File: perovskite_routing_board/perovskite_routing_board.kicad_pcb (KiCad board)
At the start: 4 copper layers, 57 x 52.2 mm, 10 parts, among them J1 G125-MH12605M4R, J2 Conn_01x08, J3 Conn_01x08, J4 Conn_01x08, J5 Conn_01x08, J6 Conn_01x08, J7 Conn_01x08

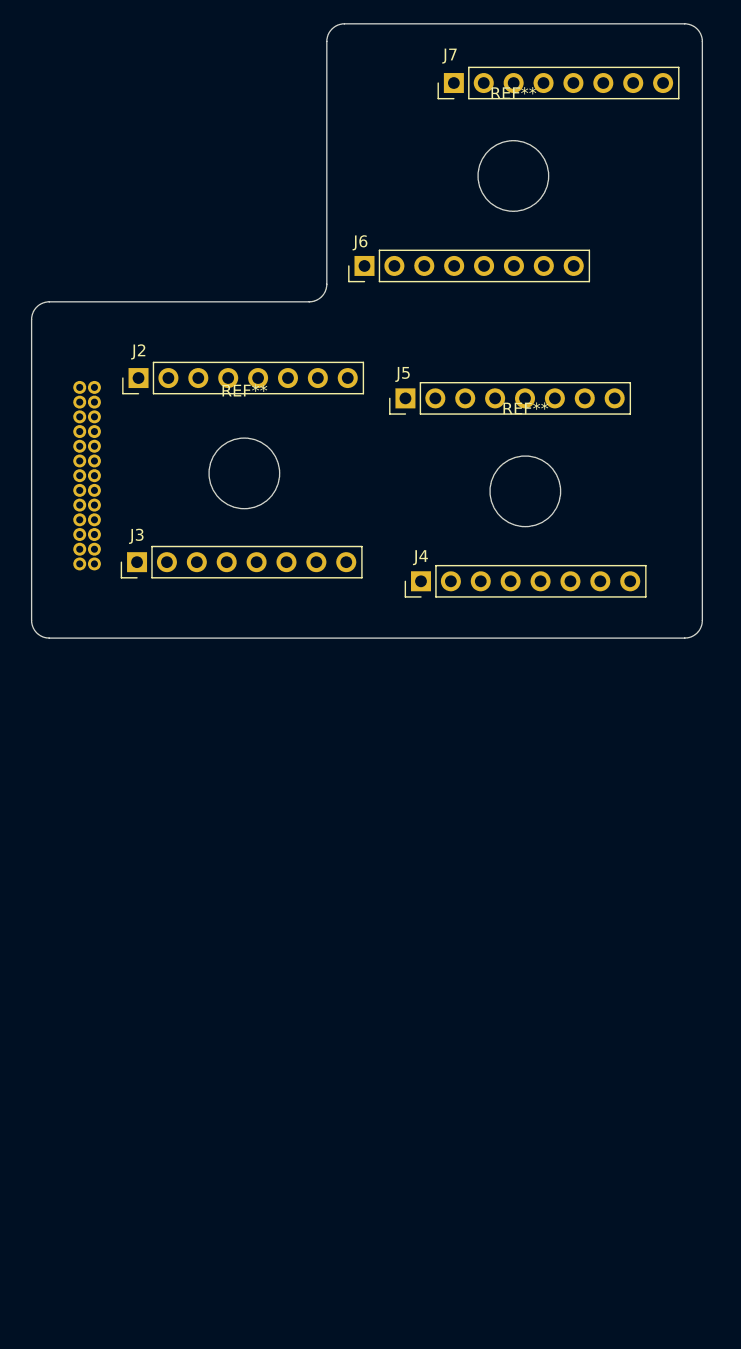
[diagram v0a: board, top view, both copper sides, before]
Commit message: update routing board
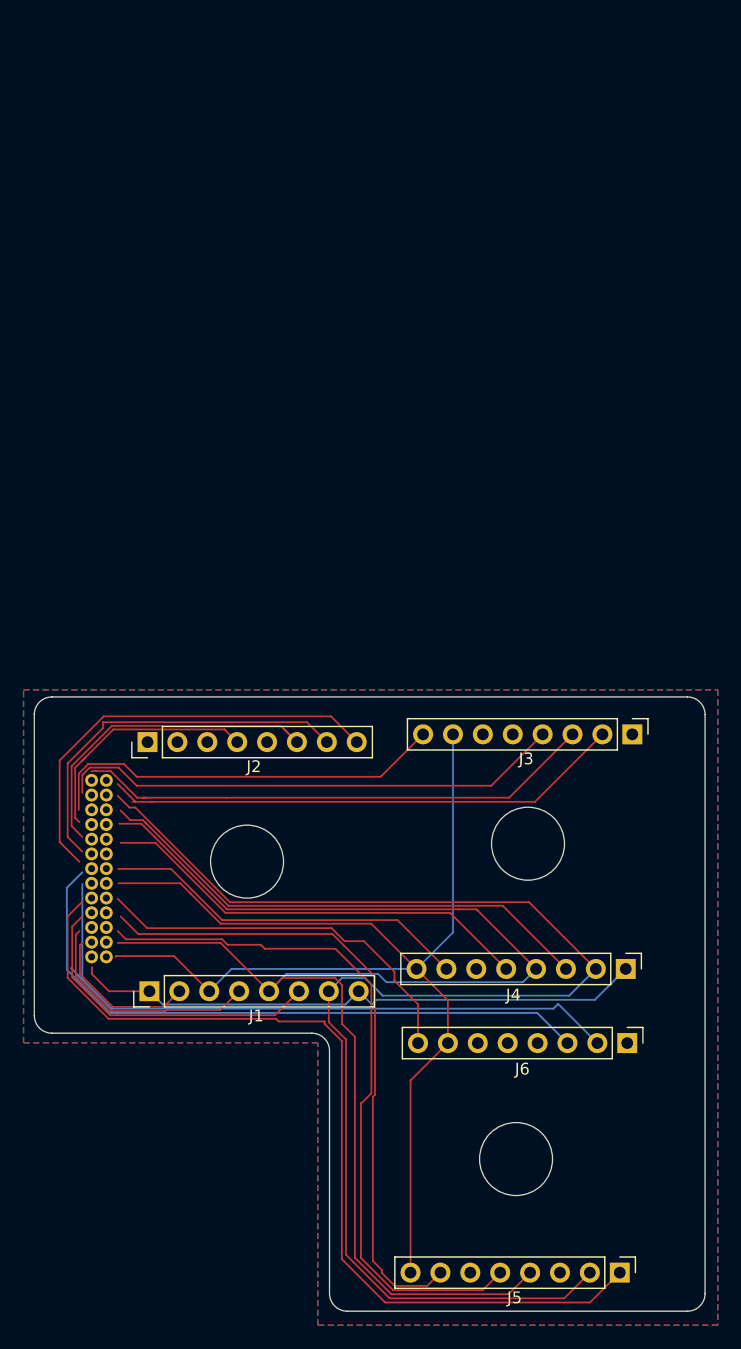
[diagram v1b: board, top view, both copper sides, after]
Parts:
- removed REF** (x3): MountingHole_6mm, MountingHole:MountingHole_6mm
- J1: value G125-MH12605M4R -> Conn_01x08; footprint MV12605M1P:G125-MV12605M1P -> Connector_PinHeader_2.54mm:PinHeader_1x08_P2.54mm_Vertical; moved to F.Cu
- J7: value Conn_01x08 -> G125-MH12605M4R; footprint Connector_PinHeader_2.54mm:PinHeader_1x08_P2.54mm_Vertical -> MV12605M1P:G125-MV12605M1P; moved to B.Cu
- moved J7 80.4 mm to (120.6, 148.0)
- moved J5 76.5 mm to (165.5, 174.9), turned to 270 degrees
- moved J6 69.7 mm to (166.1, 155.3), turned to 270 degrees
- moved J1 51.5 mm to (125.5, 150.9), turned to 90 degrees
- moved J3 44.6 mm to (166.6, 129.1), turned to 270 degrees
- moved J4 37.3 mm to (166.0, 149.0), turned to 270 degrees
- moved J2 30.9 mm to (125.4, 129.8)
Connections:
- J1 pad 1: (no net) -> CP
- J1 pad 2: (no net) -> CELL_6
- J1 pad 3: (no net) -> VDD
- J1 pad 4: (no net) -> CELL_5
- J1 pad 5: (no net) -> SDA
- J1 pad 6: (no net) -> CELL_4
- J1 pad 7: (no net) -> SCL
- J1 pad 8: (no net) -> CP
- J2 pad 1: (no net) -> GND
- J2 pad 2: (no net) -> GND
- J2 pad 3: (no net) -> GND
- J2 pad 4: (no net) -> CELL3
- J2 pad 5: (no net) -> GND
- J2 pad 6: (no net) -> CELL_2
- J2 pad 7: (no net) -> ALERT1
- J2 pad 8: (no net) -> CELL_1
- J3 pad 1: (no net) -> GND
- J3 pad 2: (no net) -> CELL_9
- J3 pad 3: (no net) -> ALERT2
- J3 pad 4: (no net) -> CELL_8
- J3 pad 5: (no net) -> GND
- J3 pad 6: (no net) -> GND
- J3 pad 7: (no net) -> VDD
- J3 pad 8: (no net) -> CELL_7
- J4 pad 1: (no net) -> CP
- J4 pad 2: (no net) -> SCL
- J4 pad 3: (no net) -> CELL_10
- J4 pad 4: (no net) -> SDA
- J4 pad 5: (no net) -> CELL_11
- J4 pad 6: (no net) -> GND
- J4 pad 7: (no net) -> CELL_12
- J4 pad 8: (no net) -> VDD
- J5 pad 1: (no net) -> CELL_16
- J5 pad 2: (no net) -> SCL
- J5 pad 3: (no net) -> GND
- J5 pad 4: (no net) -> SDA
- J5 pad 5: (no net) -> CELL_17
- J5 pad 6: (no net) -> GND
- J5 pad 7: (no net) -> CELL_18
- J5 pad 8: (no net) -> VDD
- J6 pad 1: (no net) -> GND
- J6 pad 2: (no net) -> CELL_15
- J6 pad 3: (no net) -> ALERT3
- J6 pad 4: (no net) -> GND
- J6 pad 5: (no net) -> GND
- J6 pad 6: (no net) -> CELL_14
- J6 pad 7: (no net) -> VDD
- J6 pad 8: (no net) -> CELL_13
- J7 pad 1: (no net) -> Net-(J7-Pad1)
- J7 pad 2: (no net) -> Net-(J7-Pad2)
- J7 pad 3: (no net) -> Net-(J7-Pad3)
- J7 pad 4: (no net) -> Net-(J7-Pad4)
- J7 pad 5: (no net) -> Net-(J7-Pad5)
- J7 pad 6: (no net) -> Net-(J7-Pad6)
- J7 pad 7: (no net) -> Net-(J7-Pad7)
- J7 pad 8: (no net) -> Net-(J7-Pad8)
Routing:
- net SDA: track 0.00 -> 126.7 mm
- net SCL: track 0.00 -> 117.6 mm
- net VDD: track 0.00 -> 105.4 mm
- net CELL_16: track 0.00 -> 77.4 mm
- net CELL_17: track 0.00 -> 60.7 mm
- net CELL_15: track 0.00 -> 55.9 mm
- net CELL_18: track 0.00 -> 55.2 mm
- net ALERT3: track 0.00 -> 54.0 mm
- net CP: track 0.00 -> 49.8 mm
- net CELL_9: track 0.00 -> 44.6 mm
- net ALERT2: track 0.00 -> 44.4 mm
- net CELL_10: track 0.00 -> 43.6 mm
- net CELL_8: track 0.00 -> 43.3 mm
- net CELL_11: track 0.00 -> 37.2 mm
- net CELL_1: track 0.00 -> 37.0 mm
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- added copper zone on B.Cu, net GND
- added copper zone on F.Cu, net GND
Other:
- outline, holes or cut-outs redrawn
- copper layers 4 -> 2
- net class Default: clearance 0.2 -> 0.1524; trace_width 0.25 -> 0.1524
- rule pad_to_mask_clearance: 0 -> 0.0508
- rule trace_clearance: 0.2 -> 0.1524
- rule trace_min: 0.2 -> 0.1524
- rule via_min_drill: 0.3 -> 0.254
- rule via_min_size: 0.4 -> 0.508
